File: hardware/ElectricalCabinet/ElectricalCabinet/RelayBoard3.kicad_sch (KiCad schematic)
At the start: 0 parts

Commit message: Further wiring updates
Populated 6100 Bus
Corrected number of relay boards
Added 110v outputs to relay boards and noted light positon
Uploaded light scheme to documents folder
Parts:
- added C3: 0.1uF, Capacitor_SMD:C_0805_2012Metric, symbol Device:C
- added D17, D18, D19, D20, D21, D22, D23, D24: LED, LED_SMD:LED_0805_2012Metric, symbol Device:LED
- added J6: Screw_Terminal_01x06, TerminalBlock:TerminalBlock_MaiXu_MX126-5.0-06P_1x06_P5.00mm, symbol Connector:Screw_Terminal_01x06
- added J7: Screw_Terminal_01x09, TerminalBlock:TerminalBlock_MaiXu_MX126-5.0-09P_1x09_P5.00mm, symbol Connector:Screw_Terminal_01x09
- added K17, K18, K19, K20, K21, K22, K23, K24: G3MB-202P DC5, TrafficLightLibrary:G3MB_202P_DC5, symbol TrafficLightLibrary:G3MB-202P_DC5
- added R17, R18, R19, R20, R21, R22, R23, R24: 1kΩ, Resistor_SMD:R_0805_2012Metric, symbol Device:R
- added U4: TPIC6B595N, TrafficLightLibrary:TPIC6B595N, symbol TrafficLightLibrary:TPIC6B595N
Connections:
- new net: D19.1 (K), R19.1
- new net: K19.4, R19.2, U4.6 (DRAIN2)
- new net: D22.1 (K), R22.1
- new net: K22.4, R22.2, U4.15 (DRAIN5)
- new net: D23.1 (K), R23.1
- new net: D17.2 (A), D18.2 (A), D19.2 (A), D20.2 (A), D21.2 (A), D22.2 (A), D23.2 (A), D24.2 (A), K17.3, K18.3, K19.3, K20.3, K21.3, K22.3, K23.3, K24.3
- new net: D21.1 (K), R21.1
- new net: K21.4, R21.2, U4.14 (DRAIN4)
- new net: J7.9 (Pin_9), K17.1, K18.1, K19.1, K20.1, K21.1, K22.1, K23.1, K24.1
- new net: J7.2 (Pin_2), K18.2
- new net: K18.4, R18.2, U4.5 (DRAIN1)
- new net: J6.1 (Pin_1), U4.18 (SEROUT)
- new net: C3.1, J6.2 (Pin_2), U4.10 (GND), U4.11 (GND), U4.19 (GND), U4.9 (~{G})
- new net: J6.3 (Pin_3), U4.13 (SRCK)
- new net: J6.4 (Pin_4), U4.12 (RCK)
- new net: C3.2, J6.6 (Pin_6), U4.2 (VCC), U4.8 (~{SRCLR})
- new net: D24.1 (K), R24.1
- new net: D18.1 (K), R18.1
- new net: J7.4 (Pin_4), K20.2
- new net: K20.4, R20.2, U4.7 (DRAIN3)
- new net: J7.7 (Pin_7), K23.2
- new net: K23.4, R23.2, U4.16 (DRAIN6)
- new net: D20.1 (K), R20.1
- new net: D17.1 (K), R17.1
- new net: K17.4, R17.2, U4.4 (DRAIN0)
- new net: J7.3 (Pin_3), K19.2
- new net: J7.1 (Pin_1), K17.2
- new net: J7.5 (Pin_5), K21.2
- new net: J7.6 (Pin_6), K22.2
- new net: J7.8 (Pin_8), K24.2
- new net: K24.4, R24.2, U4.17 (DRAIN7)
- new net SERIN: J6.5 (Pin_5), U4.3 (SERIN)
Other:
- note added: "RELAY MODULE 3"

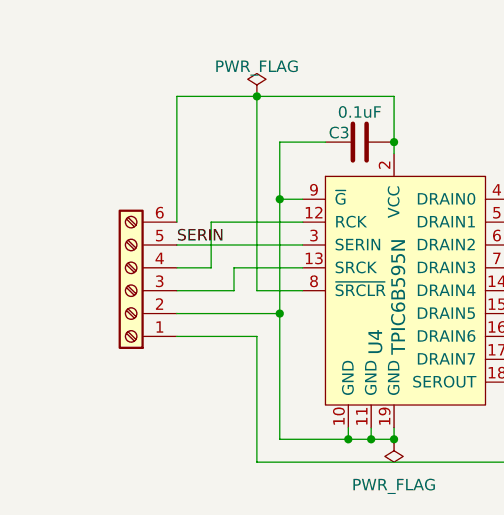
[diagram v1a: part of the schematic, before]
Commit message: Electrical Cabinet done
Electrical Cabinet done, let me know if there are any changes or mistakes.
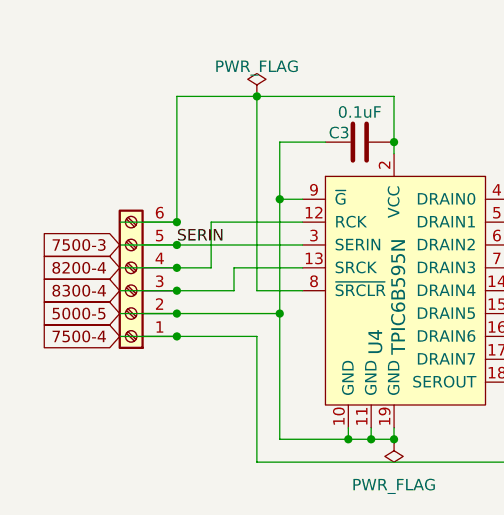
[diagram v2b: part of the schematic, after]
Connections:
- net 7500-4: now reaches J6.1 (Pin_1), U4.18 (SEROUT)
- net 5000-5: now reaches C3.1, J6.2 (Pin_2), U4.10 (GND), U4.11 (GND), U4.19 (GND), U4.9 (~{G})
- net 8300-4: now reaches J6.3 (Pin_3), U4.13 (SRCK)
- net 8200-4: now reaches J6.4 (Pin_4), U4.12 (RCK)
- net SERIN renamed 7500-3
